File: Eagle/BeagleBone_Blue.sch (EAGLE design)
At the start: 158 parts, among them M1 JST_ZH_2, M2 JST_ZH_2, M3 JST_ZH_2, M4 JST_ZH_2, Q3 MOSFET-N, U1 OSD3358, U2 CM200C-32.768KAZF-UT, U3 DMC564040R, U4 DMC564040R, U5 24LC_32AT-I/OT, Y2 445C33D24M00000

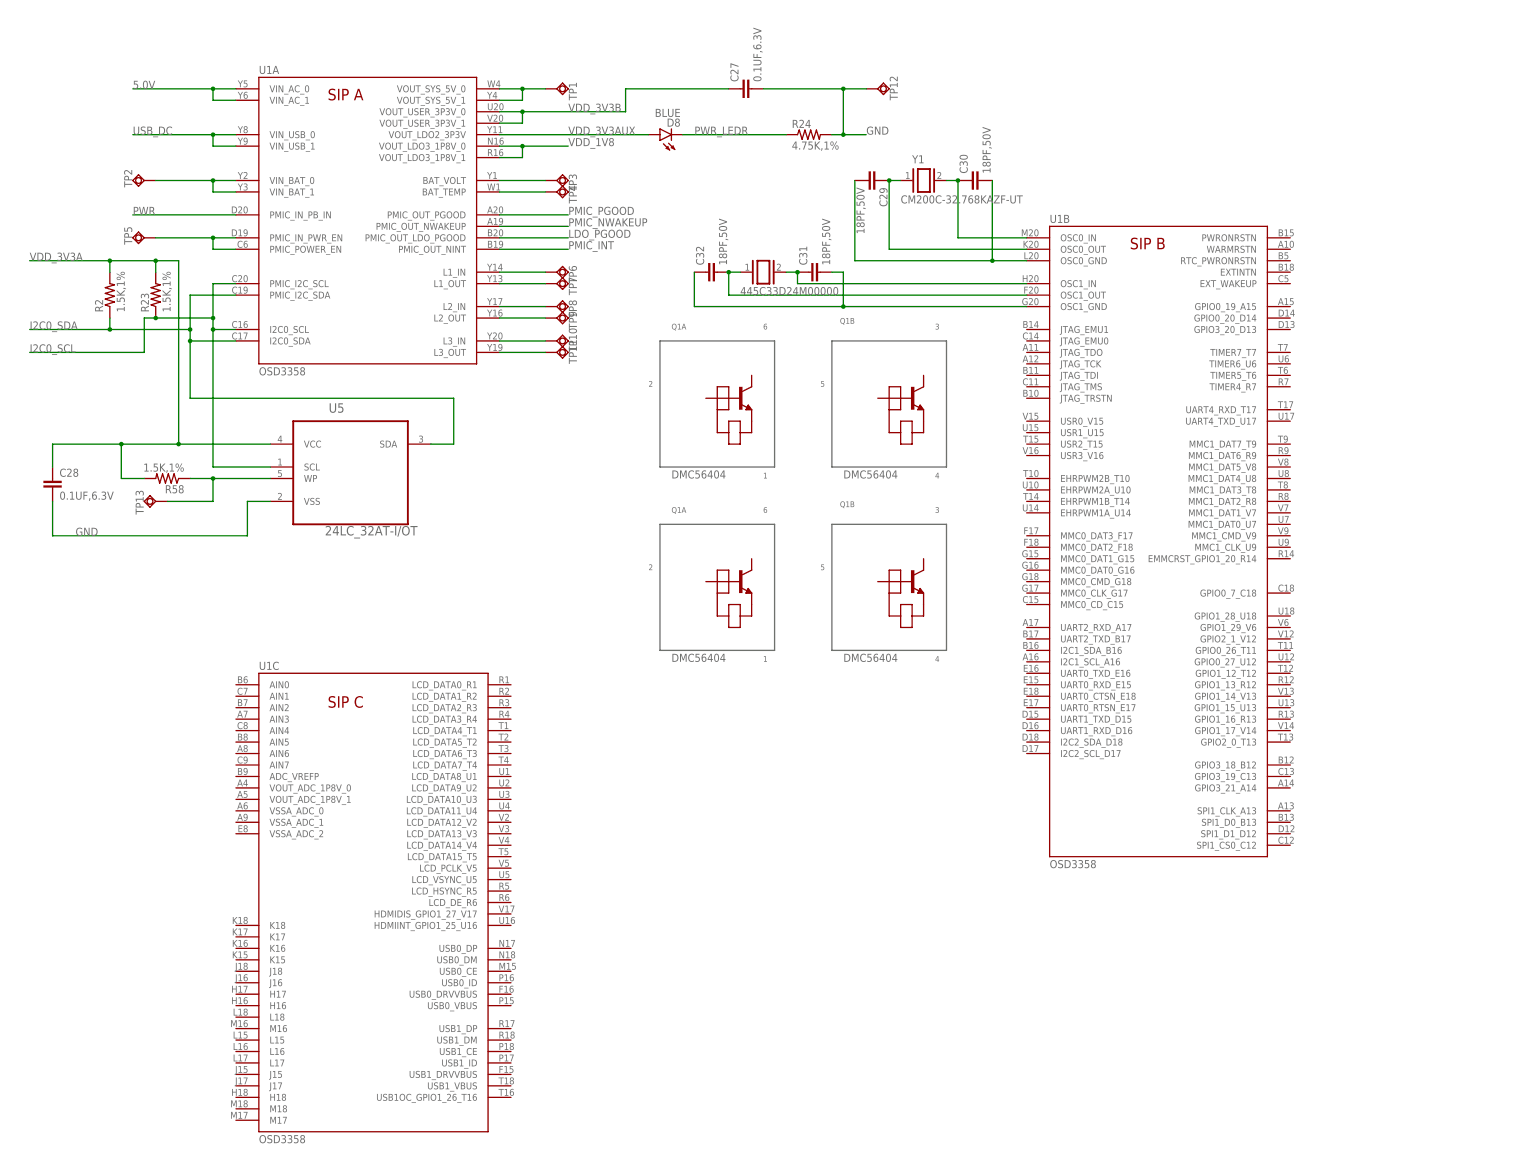
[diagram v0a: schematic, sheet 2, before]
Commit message: Some PMIC connections
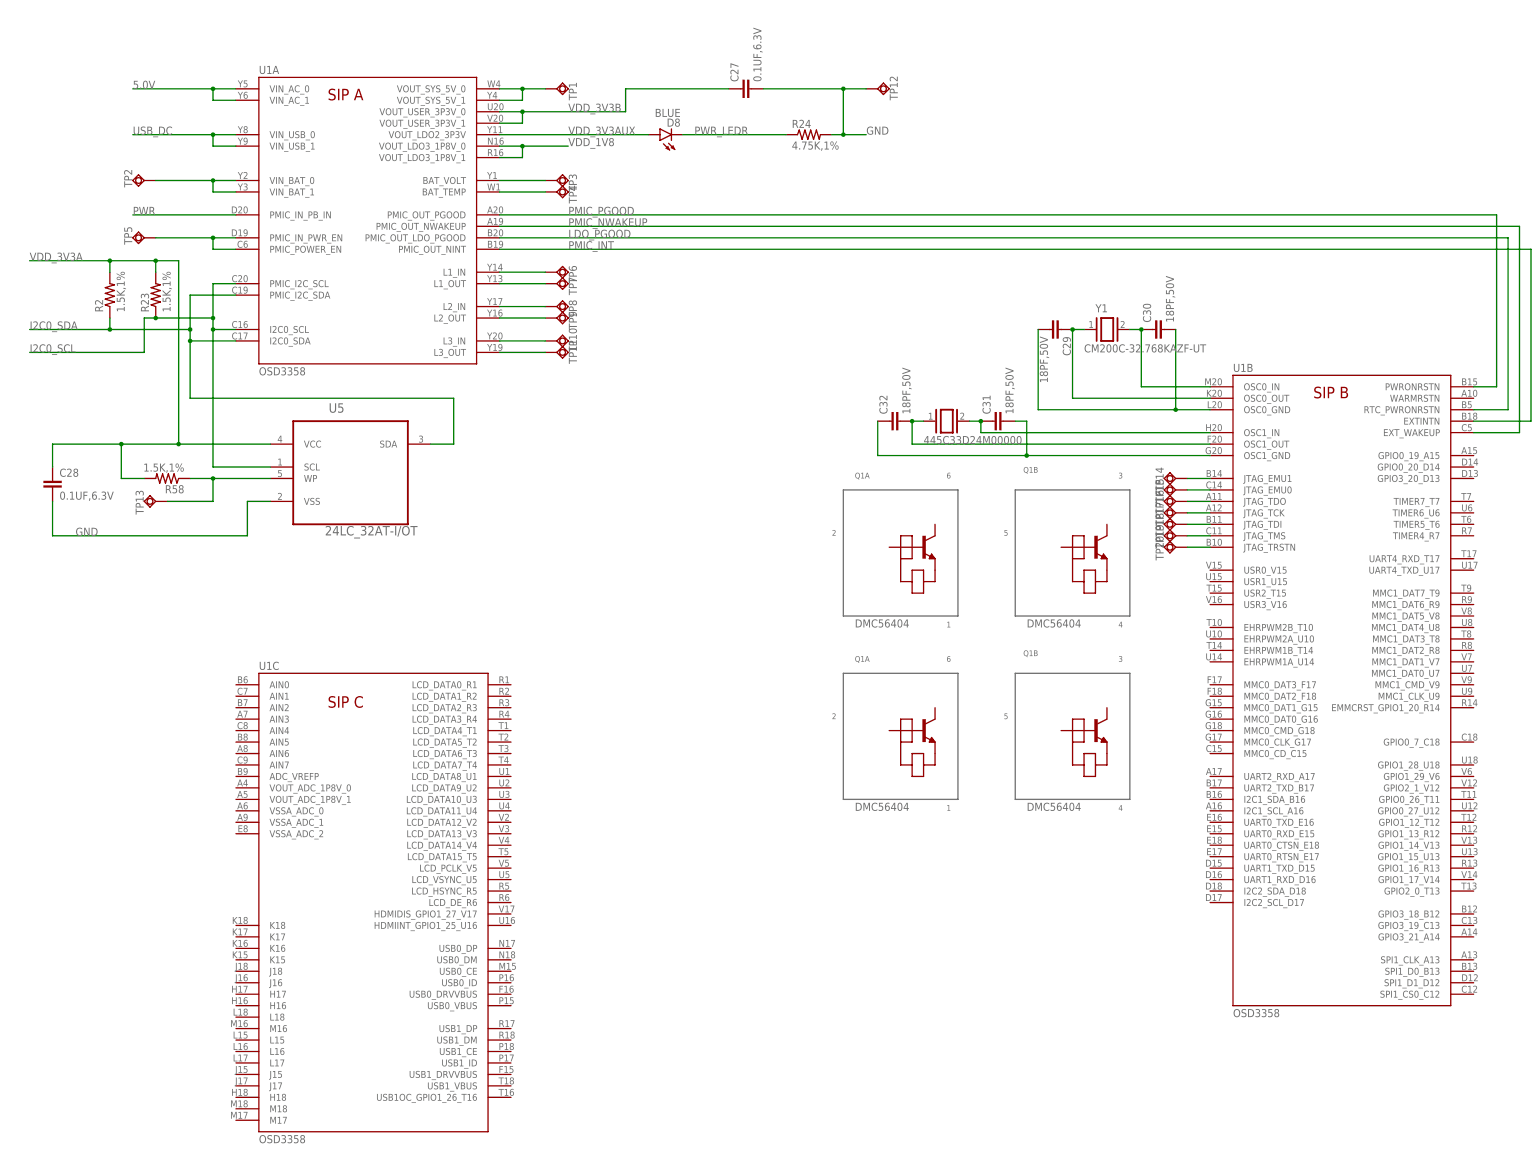
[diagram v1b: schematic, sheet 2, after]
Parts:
- added TP14, TP15, TP16, TP17, TP18, TP19, TP20: TPSQB1,27, testpad:TPSQB1,27
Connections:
- new net N$35: TP14.TP, U1B.JTAG_EMU1
- new net N$36: TP15.TP, U1B.JTAG_EMU0
- new net N$37: TP16.TP, U1B.JTAG_TDO
- new net N$39: TP17.TP, U1B.JTAG_TCK
- new net N$40: TP18.TP, U1B.JTAG_TDI
- new net N$41: TP19.TP, U1B.JTAG_TMS
- new net N$42: TP20.TP, U1B.JTAG_TRSTN
- net LDO_PGOOD: now also U1B.RTC_PWRONRSTN
- net PMIC_INT: now also U1B.EXTINTN
- net PMIC_NWAKEUP: now also U1B.EXT_WAKEUP
- net PMIC_PGOOD: now also U1B.PWRONRSTN
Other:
- moved on the sheet: C29, C30, C31, C32, U1B

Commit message: Shuffle
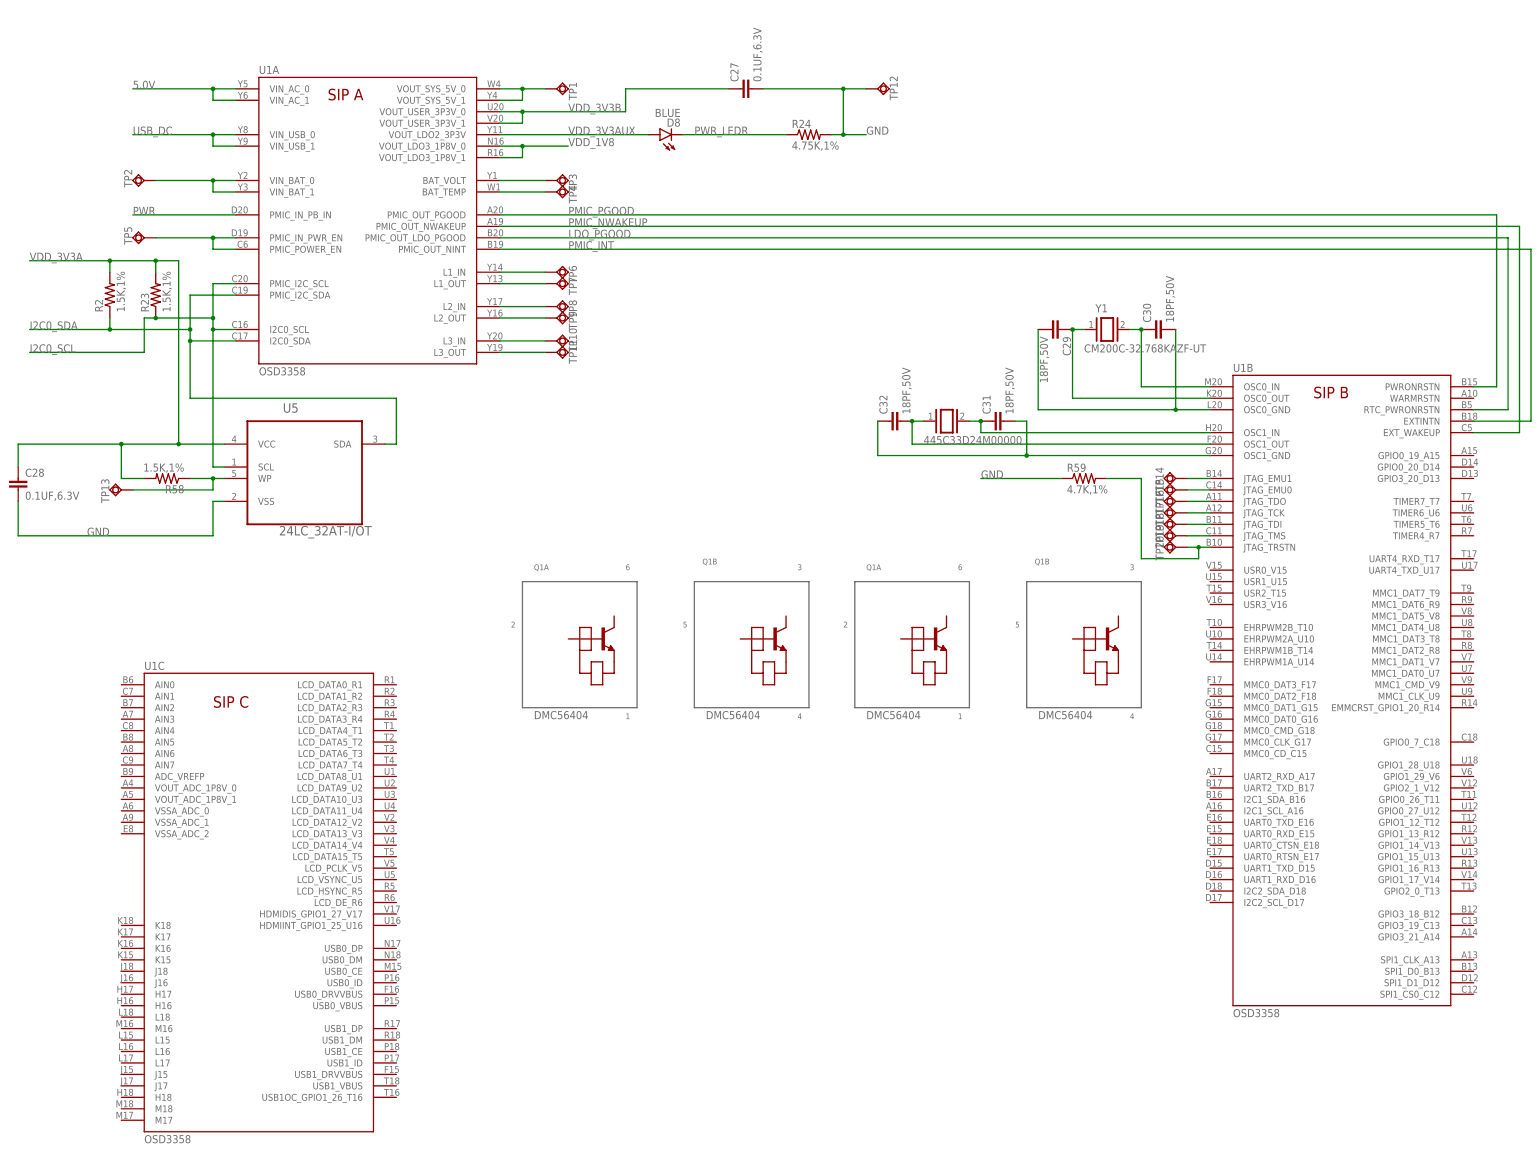
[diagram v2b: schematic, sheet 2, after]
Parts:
- added R59: 4.7K,1%, Strawson_Eagle_Lib:RESISTOR0402-RES
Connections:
- net GND: now also R59.1
- net I2C0_SCL: now also U5.SCL
- net N$42: now also R59.2
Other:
- moved on the sheet: C28, TP13, U1C, U5
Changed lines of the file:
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@@
 <part name="TP19" library="testpad" deviceset="TPSQ" device="B1,27"/>
 <part name="TP20" library="testpad" deviceset="TPSQ" device="B1,27"/>
+<part name="R59" library="Strawson_Eagle_Lib" deviceset="RESISTOR" device="0402-RES" value="4.7K,1%"/>
 </parts>
 <sheets>
@@
 <instance part="U1" gate="B" x="287.02" y="45.72"/>
 <instance part="U1" gate="A" x="71.12" y="187.96"/>
-<instance part="U1" gate="C" x="71.12" y="17.78"/>
+<instance part="U1" gate="C" x="45.72" y="17.78"/>
 <instance part="TP1" gate="G$1" x="137.16" y="248.92" rot="R90"/>
 <instance part="TP2" gate="G$1" x="45.72" y="228.6" rot="R270"/>
@@
 <instance part="C27" gate="G$1" x="180.34" y="248.92" rot="R90"/>
 <instance part="U2" gate="G$1" x="307.34" y="182.88"/>
-<instance part="U3" gate="G$1" x="236.22" y="142.24"/>
-<instance part="U4" gate="G$1" x="236.22" y="101.6"/>
-<instance part="U5" gate="A" x="73.66" y="170.18"/>
+<instance part="U3" gate="G$1" x="238.76" y="121.92"/>
+<instance part="U4" gate="G$1" x="165.1" y="121.92"/>
+<instance part="U5" gate="A" x="63.5" y="170.18"/>
 <instance part="R58" gate="G$1" x="50.8" y="162.56" rot="R180"/>
-<instance part="TP13" gate="G$1" x="48.26" y="157.48" rot="R270"/>
-<instance part="C28" gate="G$1" x="25.4" y="160.02"/>
+<instance part="TP13" gate="G$1" x="40.64" y="160.02" rot="R270"/>
+<instance part="C28" gate="G$1" x="17.78" y="160.02"/>
 <instance part="C29" gate="G$1" x="246.38" y="195.58" rot="R270"/>
 <instance part="C30" gate="G$1" x="271.78" y="195.58" rot="R90"/>
@@
 <instance part="TP19" gate="G$1" x="274.32" y="149.86" rot="R270"/>
 <instance part="TP20" gate="G$1" x="274.32" y="147.32" rot="R270"/>
+<instance part="R59" gate="G$1" x="254" y="162.56"/>
 </instances>
 <busses>
@@
 <wire x1="60.96" y1="195.58" x2="60.96" y2="165.1" width="0.1524" layer="91"/>
 <junction x="60.96" y="195.58"/>
-<wire x1="60.96" y1="165.1" x2="73.66" y2="165.1" width="0.1524" layer="91"/>
+<wire x1="60.96" y1="165.1" x2="63.5" y2="165.1" width="0.1524" layer="91"/>
+<pinref part="U5" gate="A" pin="SCL"/>
 </segment>
 </net>
@@
 <wire x1="55.88" y1="193.04" x2="55.88" y2="180.34" width="0.1524" layer="91"/>
 <junction x="55.88" y="193.04"/>
-<wire x1="55.88" y1="180.34" x2="114.3" y2="180.34" width="0.1524" layer="91"/>
-<wire x1="114.3" y1="180.34" x2="114.3" y2="170.18" width="0.1524" layer="91"/>
-<wire x1="114.3" y1="170.18" x2="109.22" y2="170.18" width="0.1524" layer="91"/>
+<wire x1="55.88" y1="180.34" x2="101.6" y2="180.34" width="0.1524" layer="91"/>
+<wire x1="101.6" y1="180.34" x2="101.6" y2="170.18" width="0.1524" layer="91"/>
+<wire x1="101.6" y1="170.18" x2="99.06" y2="170.18" width="0.1524" layer="91"/>
 <pinref part="U5" gate="A" pin="SDA"/>
 </segment>
@@
 <wire x1="53.34" y1="210.82" x2="53.34" y2="170.18" width="0.1524" layer="91"/>
 <pinref part="U5" gate="A" pin="VCC"/>
-<wire x1="53.34" y1="170.18" x2="73.66" y2="170.18" width="0.1524" layer="91"/>
+<wire x1="53.34" y1="170.18" x2="63.5" y2="170.18" width="0.1524" layer="91"/>
 <wire x1="53.34" y1="170.18" x2="40.64" y2="170.18" width="0.1524" layer="91"/>
 <junction x="53.34" y="170.18"/>
@@
 <wire x1="40.64" y1="162.56" x2="45.72" y2="162.56" width="0.1524" layer="91"/>
 <pinref part="C28" gate="G$1" pin="1"/>
-<wire x1="40.64" y1="170.18" x2="25.4" y2="170.18" width="0.1524" layer="91"/>
-<wire x1="25.4" y1="170.18" x2="25.4" y2="165.1" width="0.1524" layer="91"/>
+<wire x1="40.64" y1="170.18" x2="17.78" y2="170.18" width="0.1524" layer="91"/>
+<wire x1="17.78" y1="170.18" x2="17.78" y2="165.1" width="0.1524" layer="91"/>
 <junction x="40.64" y="170.18"/>
 </segment>
@@
 <segment>
 <pinref part="U5" gate="A" pin="VSS"/>
-<wire x1="73.66" y1="157.48" x2="68.58" y2="157.48" width="0.1524" layer="91"/>
-<wire x1="68.58" y1="157.48" x2="68.58" y2="149.86" width="0.1524" layer="91"/>
-<wire x1="68.58" y1="149.86" x2="25.4" y2="149.86" width="0.1524" layer="91"/>
+<wire x1="63.5" y1="157.48" x2="60.96" y2="157.48" width="0.1524" layer="91"/>
+<wire x1="60.96" y1="157.48" x2="60.96" y2="149.86" width="0.1524" layer="91"/>
+<wire x1="60.96" y1="149.86" x2="17.78" y2="149.86" width="0.1524" layer="91"/>
 <pinref part="C28" gate="G$1" pin="2"/>
-<wire x1="25.4" y1="149.86" x2="25.4" y2="157.48" width="0.1524" layer="91"/>
-<label x="30.48" y="149.86" size="1.778" layer="95"/>
+<wire x1="17.78" y1="149.86" x2="17.78" y2="157.48" width="0.1524" layer="91"/>
+<label x="33.02" y="149.86" size="1.778" layer="95"/>
+</segment>
+<segment>
+<pinref part="R59" gate="G$1" pin="1"/>
+<wire x1="248.92" y1="162.56" x2="231.14" y2="162.56" width="0.1524" layer="91"/>
+<label x="231.14" y="162.56" size="1.778" layer="95"/>
 </segment>
 </net>
@@
 <wire x1="55.88" y1="162.56" x2="60.96" y2="162.56" width="0.1524" layer="91"/>
 <pinref part="TP13" gate="G$1" pin="TP"/>
-<wire x1="60.96" y1="162.56" x2="73.66" y2="162.56" width="0.1524" layer="91"/>
-<wire x1="50.8" y1="157.48" x2="60.96" y2="157.48" width="0.1524" layer="91"/>
-<wire x1="60.96" y1="157.48" x2="60.96" y2="162.56" width="0.1524" layer="91"/>
+<wire x1="60.96" y1="162.56" x2="63.5" y2="162.56" width="0.1524" layer="91"/>
+<wire x1="43.18" y1="160.02" x2="60.96" y2="160.02" width="0.1524" layer="91"/>
+<wire x1="60.96" y1="160.02" x2="60.96" y2="162.56" width="0.1524" layer="91"/>
 <junction x="60.96" y="162.56"/>
 </segment>
@@
 <segment>
 <pinref part="U1" gate="B" pin="JTAG_TRSTN"/>
-<wire x1="276.86" y1="147.32" x2="281.94" y2="147.32" width="0.1524" layer="91"/>
+<wire x1="276.86" y1="147.32" x2="279.4" y2="147.32" width="0.1524" layer="91"/>
 <pinref part="TP20" gate="G$1" pin="TP"/>
-</segment>
-</net>
+<pinref part="R59" gate="G$1" pin="2"/>
+<wire x1="279.4" y1="147.32" x2="281.94" y2="147.32" width="0.1524" layer="91"/>
+<wire x1="259.08" y1="162.56" x2="266.7" y2="162.56" width="0.1524" layer="91"/>
+<wire x1="266.7" y1="162.56" x2="266.7" y2="144.78" width="0.1524" layer="91"/>
+<wire x1="266.7" y1="144.78" x2="279.4" y2="144.78" width="0.1524" layer="91"/>
+<wire x1="279.4" y1="144.78" x2="279.4" y2="147.32" width="0.1524" layer="91"/>
+<junction x="279.4" y="147.32"/>
+</segment>
+</net>
